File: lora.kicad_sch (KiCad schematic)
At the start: 29 parts, among them J5 Conn_Coaxial, Q1 2N7002, U3 E22P-915M30S

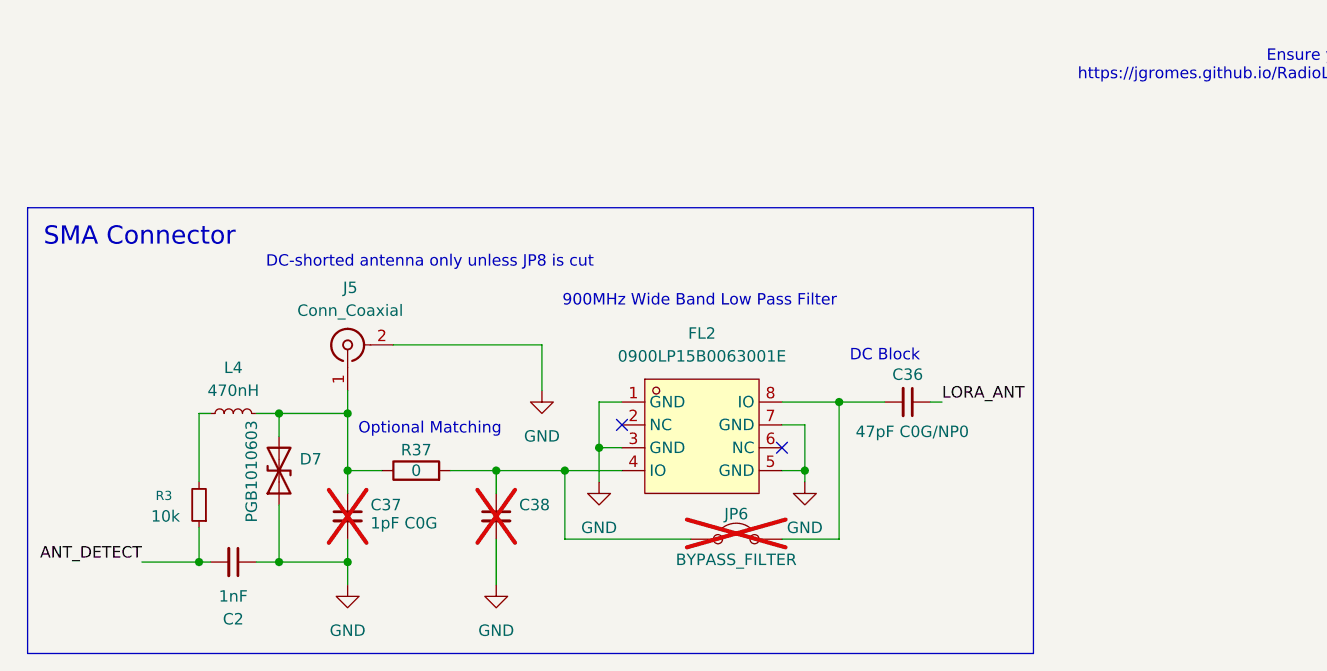
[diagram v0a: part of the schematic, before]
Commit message: usb-org
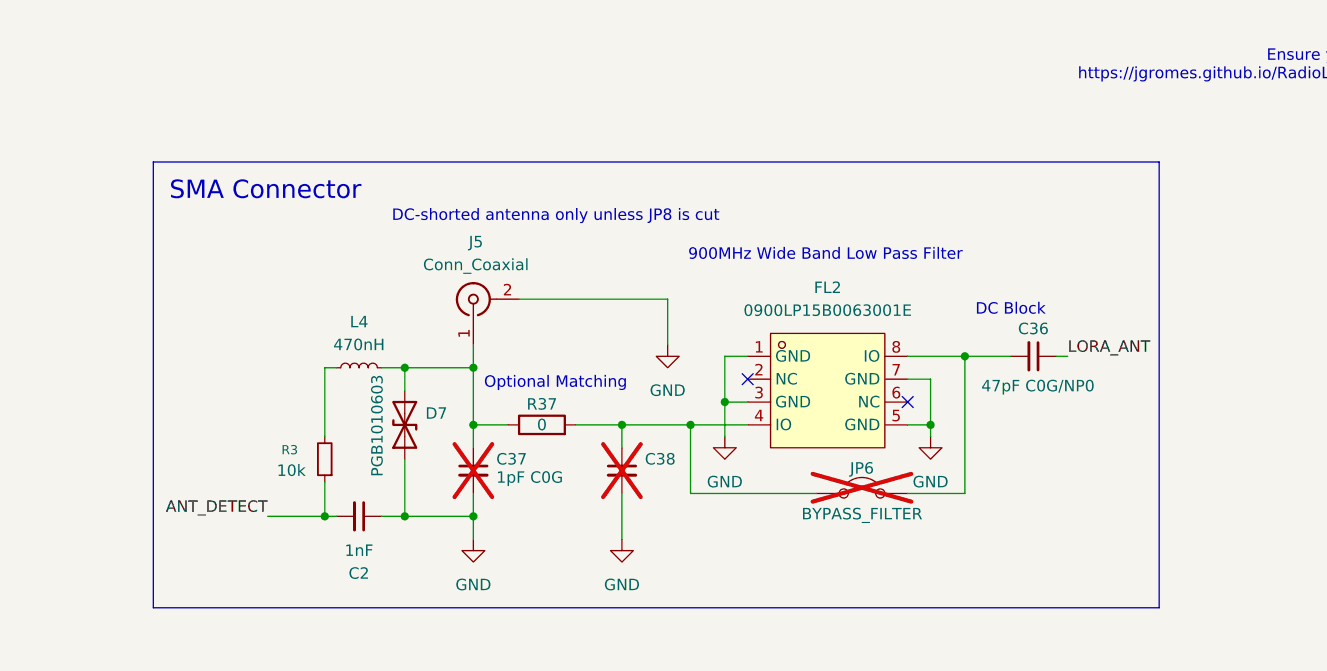
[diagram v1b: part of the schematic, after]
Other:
- moved on the sheet: C2, C36, C37, C38, D7, FL2, J5, JP6, L4, R3, R37
